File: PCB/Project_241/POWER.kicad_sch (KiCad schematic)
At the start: 5 parts, among them J6 BATT_CONN, U7 RT9013

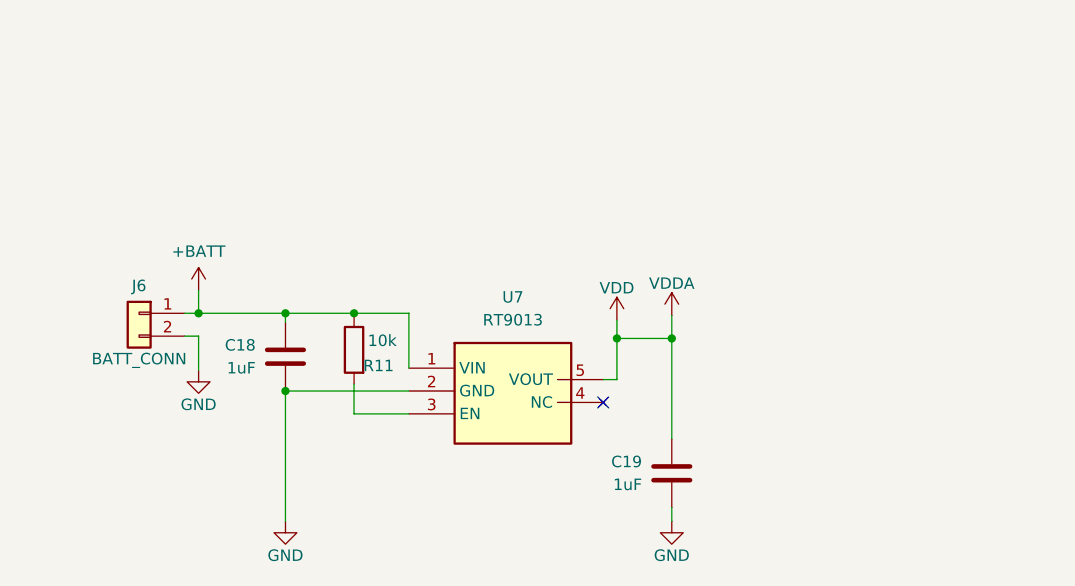
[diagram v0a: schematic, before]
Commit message: update gerber
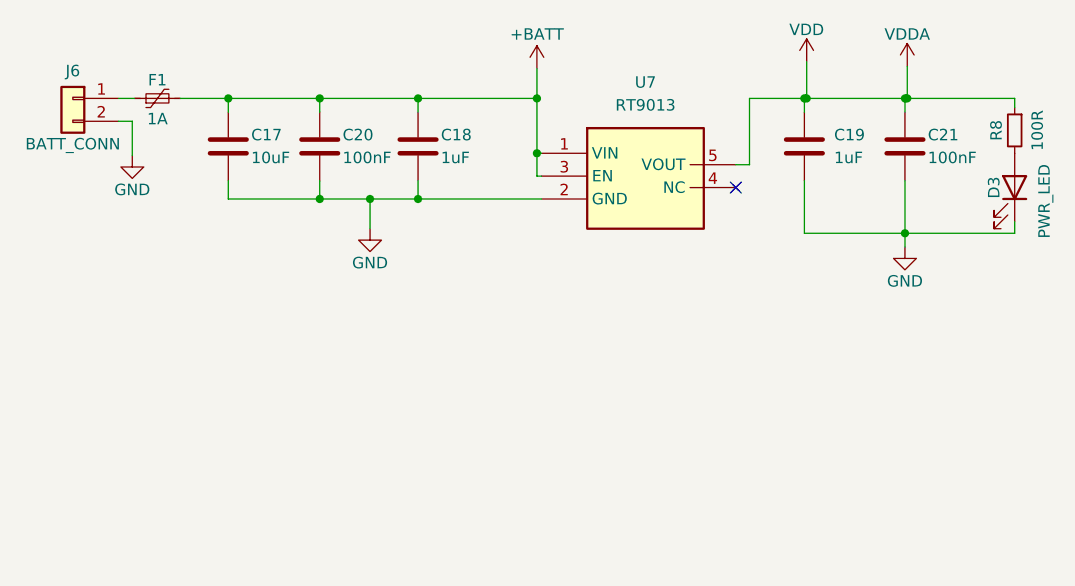
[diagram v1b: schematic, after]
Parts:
- removed R11: 10k, Resistor_SMD:R_0603_1608Metric, symbol Device:R
- added C17: 10uF, Capacitor_SMD:C_0603_1608Metric, symbol Device:C
- added C20, C21: 100nF, Capacitor_SMD:C_0603_1608Metric, symbol Device:C
- added D3: PWR_LED, LED_SMD:LED_0603_1608Metric, symbol Device:LED
- added F1: 1A, Fuse:Fuse_0805_2012Metric, symbol Device:Polyfuse_Small
- added R8: 100R, Resistor_SMD:R_0603_1608Metric, symbol Device:R_Small
- J6: footprint IVSFootprint:XH_2P_2.54mm_Horizontal_SMD -> IVSFootprint:XH 2.54 2Pin Female
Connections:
- net +BATT: now also U7.3 (EN), C17.1, C20.1, F1.2; no longer J6.1 (Pin_1)
- net GND: now also C17.2, C20.2, C21.2, D3.1 (K)
- net VDD: now also C21.1, R8.1
- new net: D3.2 (A), R8.2
- new net: F1.1, J6.1 (Pin_1)
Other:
- moved on the sheet: C18, C19, J6, U7
